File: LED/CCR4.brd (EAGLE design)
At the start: 72.4 x 35.6 mm, 13 parts, among them Q2 STP11NM60ND, Q3 ST13003, X1 MKDSN1,5/2-5,08, X3 MKDSN1,5/2-5,08

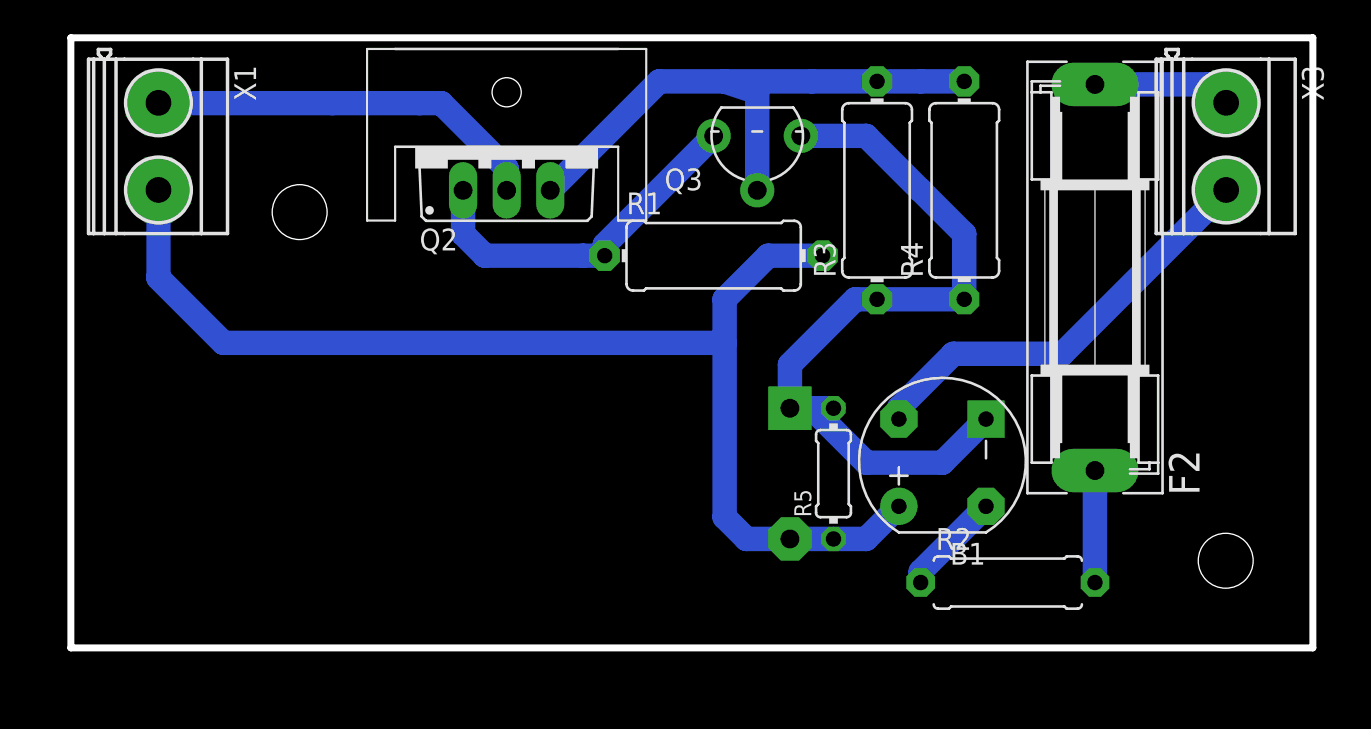
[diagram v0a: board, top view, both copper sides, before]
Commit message: _
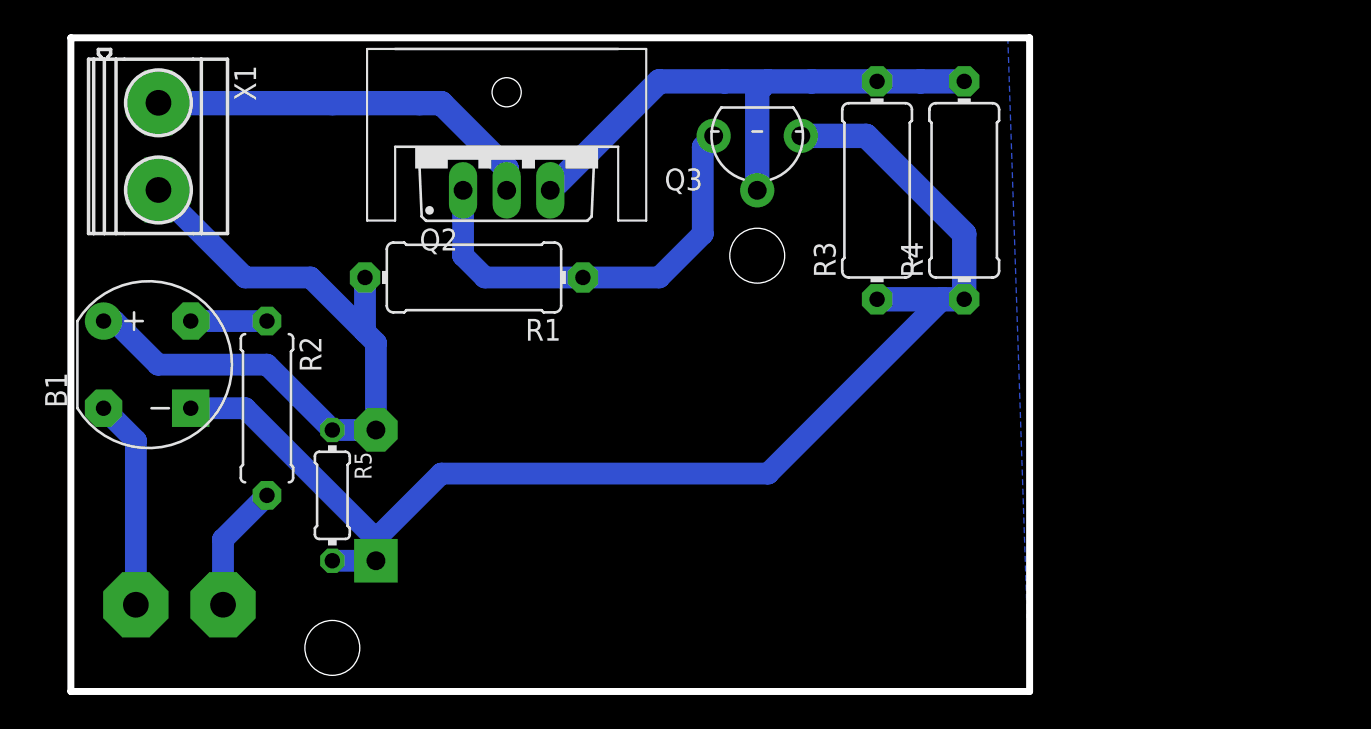
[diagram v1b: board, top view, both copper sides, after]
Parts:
- removed F2: FUSESH22,5, fuse:SH22,5
- moved X3 66.5 mm to (71.1, 2.54), flipped to the bottom, turned to 180 degrees
- moved B1 46.7 mm to (69.2, 16.5), turned to 0 degrees
- moved R2 44.4 mm to (76.2, 14.0), turned to 270 degrees
- moved R5 29.2 mm to (80.0, 8.89), turned to 270 degrees
- moved U$1 24.2 mm to (82.5, 8.89), turned to 0 degrees
- moved R1 14.0 mm to (88.3, 21.6), turned to 180 degrees
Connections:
- removed net N$8: F2.1, R2.2
- net N$2: now also R2.1; no longer X3.2
- net N$3: now also R2.2, X3.2; no longer B1.AC2, R2.1
- net N$4: now also B1.AC2; no longer F2.2
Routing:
- net N$9: track 46.3 -> 77.4 mm
- net N$1: track 70.6 -> 43.2 mm
- net N$2: track 25.0 -> 4.44 mm
- net N$8: track 6.53 -> 0.00 mm
- net N$7: track 20.9 -> 25.3 mm
- net N$4: track 8.09 -> 12.2 mm
- net N$3: track 6.02 -> 7.44 mm
- net N$6: track 34.5 -> 33.7 mm
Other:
- board size 72.4 x 35.6 mm -> 55.9 x 38.1 mm
